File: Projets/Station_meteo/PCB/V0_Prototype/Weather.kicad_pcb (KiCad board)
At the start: 2 copper layers, 94.4 x 77 mm, 161 parts, among them J1 SolderJumper_2_Bridged, J10 SolderJumper_2_Bridged, J11 SolderJumper_2_Bridged, J12 SolderJumper_2_Bridged, J13 SolderJumper_2_Bridged, J14 SolderJumper_2_Bridged, J15 SolderJumper_2_Bridged, J16 SolderJumper_2_Bridged, J17 SolderJumper_2_Bridged, J18 SolderJumper_2_Bridged, J19 SolderJumper_2_Bridged, J2 SolderJumper_2_Bridged, J20 SolderJumper_2_Bridged, J21 SolderJumper_2_Bridged, J22 SolderJumper_2_Bridged, J23 SolderJumper_2_Bridged, J24 Anemometer, J25 KF128-2.54_2P, J26 Panel, J27 132415, J28 SolderJumper_2_Bridged, J29 USB_C_Receptacle_USB2.0_16P, J3 SolderJumper_2_Bridged, J30 KF128-2.54_2P, J31 Wind_Direction, J32 Water_Level, J33 Screw_Terminal_01x04, J34 SolderJumper_2_Bridged, J4 SolderJumper_2_Bridged, J5 SolderJumper_2_Bridged, J6 SolderJumper_2_Bridged, J7 SolderJumper_2_Bridged, J8 SolderJumper_2_Bridged, J9 SolderJumper_2_Bridged, Q1 CJ3401, Q2 2N7002H, Q3 CJ3401, Q4 2N7002H, Q5 CJ3401, Q6 2N7002H, SW1 PB_SMD_12V_50MA_6MM_6MM, SW2 PB_SMD_12V_50MA_6MM_6MM, T1 TP, T10 TP, T11 TP, T14 TP, T15 TP, T16 TP, T17 TP, T18 TP, T19 TP, T2 TP, T20 TP, T3 TP, T4 TP, T5 TP, T6 TP, T7 TP, T8 TP, T9 TP, U1 ATMEGA-328P, U10 USBLC6-2P6, U11 CH340G, U12 AMS1117-3.3, U13 DS3231M, U2 LM358DR, U3 74HC123D, U6 LM317_SOT-223, U7 BL8530, U8 NRF24L01, U9 NEO-M8M, Y1 16MHz, Y2 16MHz, Y3 12MHz

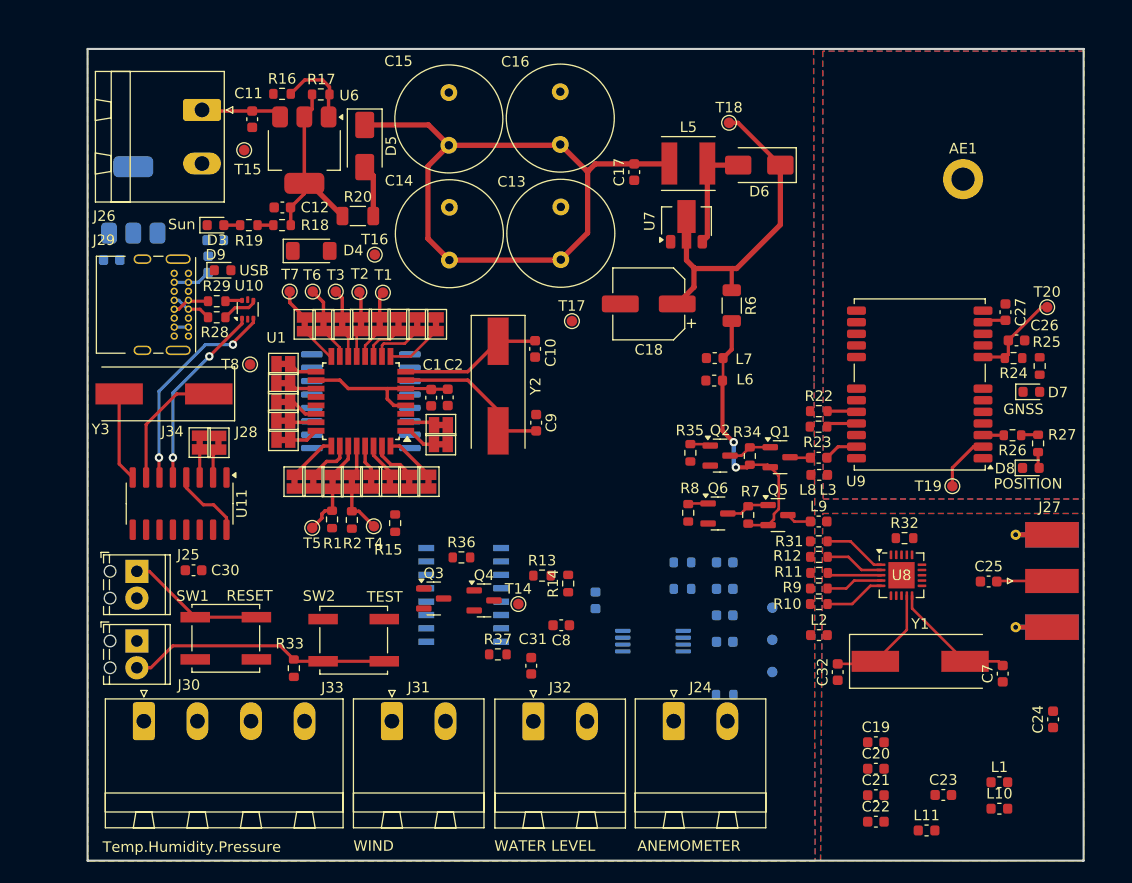
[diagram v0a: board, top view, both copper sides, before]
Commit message: Update PCB
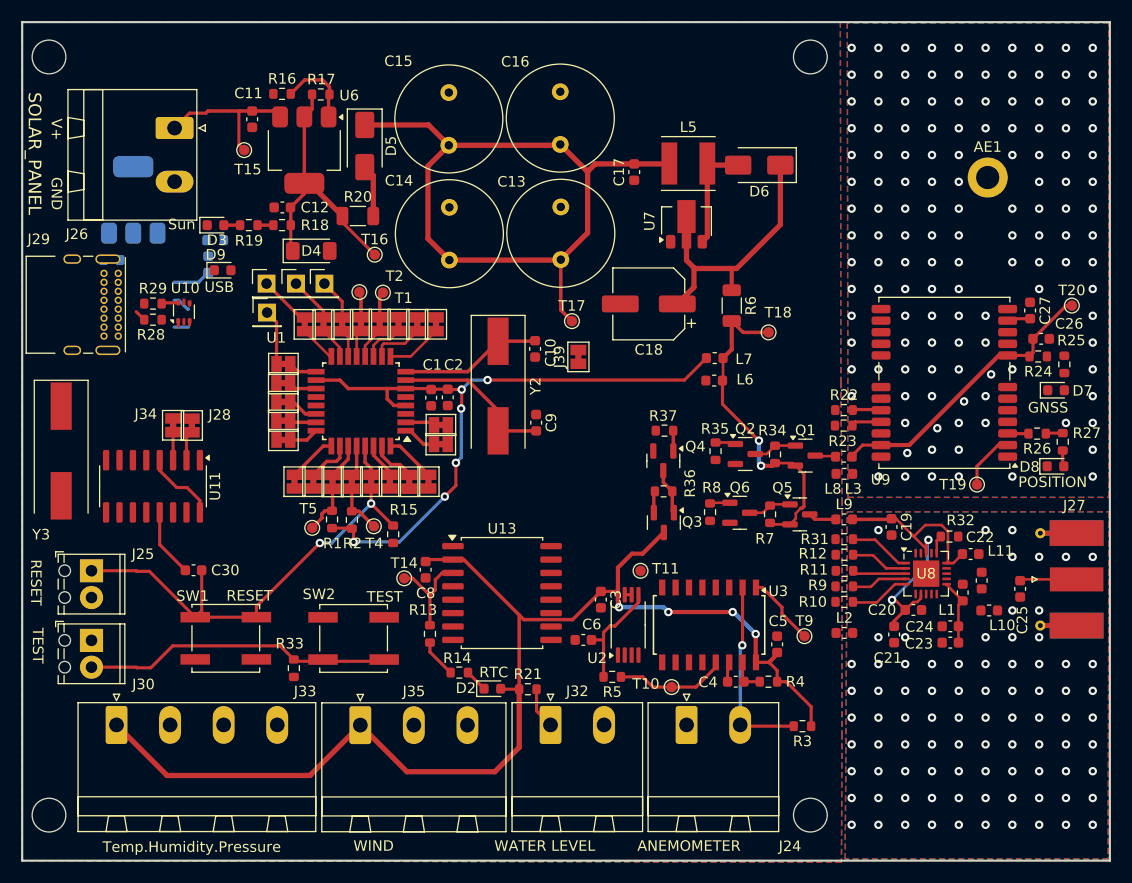
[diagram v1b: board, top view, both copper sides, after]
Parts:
- removed C31: 100nF, Capacitor_SMD:C_0603_1608Metric
- removed C32, C7: 22pF, Capacitor_SMD:C_0603_1608Metric
- removed T3, T6, T7, T8: TP, TestPoint:TestPoint_Pad_D1.0mm
- removed Y1: 16MHz, Crystal:Crystal_SMD_HC49-SD
- added H1: MountingHole_Pad, MountingHole:MountingHole_3.2mm_M3, F.Cu at (117.9, 64.8)
- added H2: MountingHole_Pad, MountingHole:MountingHole_3.2mm_M3, F.Cu at (45.7, 64.8)
- added H3: MountingHole_Pad, MountingHole:MountingHole_3.2mm_M3, F.Cu at (45.7, 136.7)
- added H4: MountingHole_Pad, MountingHole:MountingHole_3.2mm_M3, F.Cu at (117.9, 136.7)
- added J35: Screw_Terminal_01x03, Connector_Phoenix_MSTB:PhoenixContact_MSTBA_2,5_3-G-5,08_1x03_P5.08mm_Horizontal, F.Cu at (75.2, 128.1)
- added J36: Conn_01x01_Pin, Connector_PinHeader_2.54mm:PinHeader_1x01_P2.54mm_Vertical, F.Cu at (66.3, 86.3)
- added J37: Conn_01x01_Pin, Connector_PinHeader_2.54mm:PinHeader_1x01_P2.54mm_Vertical, F.Cu at (66.4, 89.0)
- added J38: Conn_01x01_Pin, Connector_PinHeader_2.54mm:PinHeader_1x01_P2.54mm_Vertical, F.Cu at (71.8, 86.3)
- added J39: SolderJumper_2_Bridged, Jumper:SolderJumper-2_P1.3mm_Bridged_Pad1.0x1.5mm, F.Cu at (95.9, 93.2)
- added R21: 100k, Resistor_SMD:R_0603_1608Metric, F.Cu at (91.1, 124.7)
- C3, C4, C5, C6, D2, R3, R4, R5, T10, T11, T9, U13, U2, U3: moved to F.Cu
- J31: value Wind_Direction -> Conn_01x01_Pin; footprint Connector_Phoenix_MSTB:PhoenixContact_MSTBA_2,5_2-G-5,08_1x02_P5.08mm_Horizontal -> Connector_PinHeader_2.54mm:PinHeader_1x01_P2.54mm_Vertical
- moved J31 42.5 mm to (69.1, 86.3)
- moved C22 26.9 mm to (133.1, 111.9)
- moved R37 26.4 mm to (104.1, 100.2), turned to 180 degrees
- moved L11 24.3 mm to (134.2, 114.4), turned to 90 degrees
- moved U3 23.4 mm to (108.3, 118.6), turned to -90 degrees
- moved Q3 23.0 mm to (104.0, 108.9), turned to -90 degrees
- moved U13 22.6 mm to (88.7, 115.6), turned to 0 degrees
- moved Q4 21.5 mm to (104.0, 103.1), turned to -90 degrees
- moved C19 20.5 mm to (125.6, 109.3), turned to -90 degrees
- moved T18 20.2 mm to (113.9, 90.9)
- moved R36 20.2 mm to (104.0, 106.0), turned to 180 degrees
- moved L10 18.8 mm to (134.9, 117.2)
- moved L1 18.3 mm to (132.3, 115.5), turned to 90 degrees
- moved T11 15.8 mm to (101.8, 113.5), turned to 0 degrees
- moved C20 15.5 mm to (127.7, 117.2)
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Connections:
- net /Power/Vcap renamed Net-(D5-K)
- net /RTC/+3.3V renamed /Interfaces/+3.3V
- J11 pad 2: /MCU/PC2-A2 -> /Interfaces/Direction
- J18 pad 2: /MCU/PD2-D2-(INT0) -> /Interfaces/Water_Level
- J30 pad 2: /MCU/PB2-D10~ -> /MCU/PD3-D3-(INT1)~
- J31 pad 1: unconnected-(J31-Pin_1-Pad1) -> /MCU/MOSI
- J32 pad 1: unconnected-(J32-Pin_1-Pad1) -> /Interfaces/Water_Level
- J32 pad 2: unconnected-(J32-Pin_2-Pad2) -> GND
- L7 pad 2: /+3.3V_MCU -> /MCU/+VCC
- R33 pad 1: /User_Buttons/VCC -> /+3.3V_MCU
- R33 pad 2: /MCU/PB2-D10~ -> /MCU/PD3-D3-(INT1)~
- SW2 pad 2: /MCU/PB2-D10~ -> /MCU/PD3-D3-(INT1)~
- T9 pad 1: /WIND/Simulation -> /MCU/PB1-D9~
- U3 pad 1: /WIND/Simulation -> /MCU/PB1-D9~
- U8 pad 10: /NRF24/XTAL1/XTAl_1 -> /NRF24/XTAl_1
- U8 pad 9: /NRF24/XTAL1/XTAl_2 -> /NRF24/XTAl_2
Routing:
- net /Interfaces/+3.3V: track 0.00 -> 118.1 mm, vias 0 -> 4
- net /MCU/+VCC: track 15.9 -> 66.1 mm, vias 0 -> 6
- net /NRF24/+3.3V: track 2.39 -> 34.6 mm, vias 0 -> 2
- net /RESET: track 13.1 -> 42.5 mm, vias 0 -> 2
- net /MCU/PD3-D3-(INT1)~: track 0.00 -> 29.3 mm
- net /MCU/PB2-D10~: track 27.6 -> 3.91 mm
- net /Programming/D-: track 20.3 -> 0.47 mm, vias 2 -> 0
- net Net-(J24-Pin_2): track 0.00 -> 18.3 mm, vias 0 -> 1
- net /Programming/D+: track 17.8 -> 0.51 mm, vias 2 -> 0
- net /GNSS/+3.3V: track 14.1 -> 29.6 mm
- net Net-(U11-XI): track 12.2 -> 0.00 mm
- net /NRF24/XTAL1/XTAl_1: track 12.0 -> 0.00 mm
- net /NRF24/XTAL1/XTAl_2: track 11.1 -> 0.00 mm
- net Net-(U3A-Q): track 0.00 -> 10.6 mm
- net Net-(U2B-+): track 0.00 -> 10.6 mm
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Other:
- board size 94.4 x 77 mm -> 103.1 x 79.5 mm
- board text added: "${REFERENCE}"
- board text added: "GND"
- board text added: "RTC"
- board text added: "SOLAR_PANEL"
- board text added: "V+"
